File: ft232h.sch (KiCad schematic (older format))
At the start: 50 parts, among them CON1 USB-MINI-B, IC1 V_REG_LM1117SOT223, P3 CONN_13, P4 CONN_13, P5 CONN_4, P6 CONN_1, P7 CONN_6, Q1 BCX51, Q2 BCX51, U3 FT232H, U5 93LC56CX-X/SN_SOIC8-N_MC, X1 12MHz

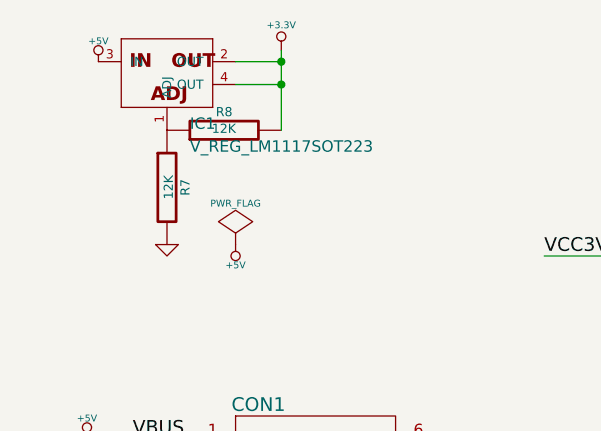
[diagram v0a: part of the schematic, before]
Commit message: ftdi done + breakout done + silk done
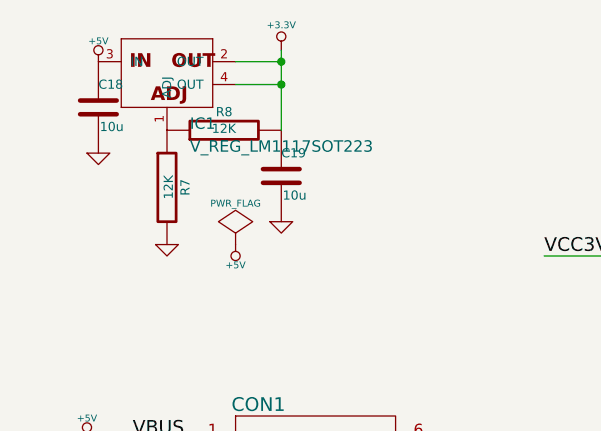
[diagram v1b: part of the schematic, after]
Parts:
- added C18, C19: 10u, ~, symbol C
